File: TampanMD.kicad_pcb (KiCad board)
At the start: 2 copper layers, 50 x 50 mm, 93 parts, among them J1 Conn_01x10, U1 F2800132RHBR, U10 BSC009NE2LS, U11 AMC1301DWVR, U12 TLV62130, U2 UCC27211DRMR, U3 UCC27211DRMR, U4 UCC27211DRMR, U5 BSC009NE2LS, U6 BSC009NE2LS, U7 BSC009NE2LS, U8 BSC009NE2LS, U9 BSC009NE2LS, Y1 X322520MSB4SI

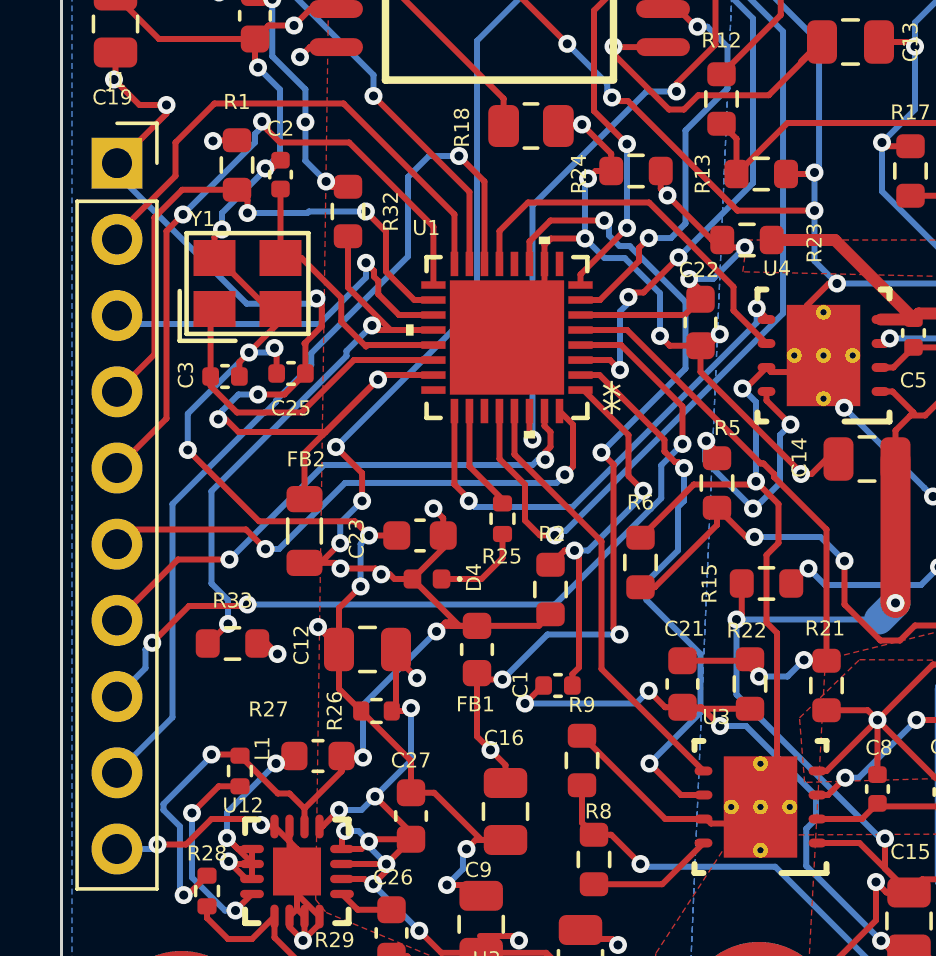
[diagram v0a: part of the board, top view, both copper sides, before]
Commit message: done i guess
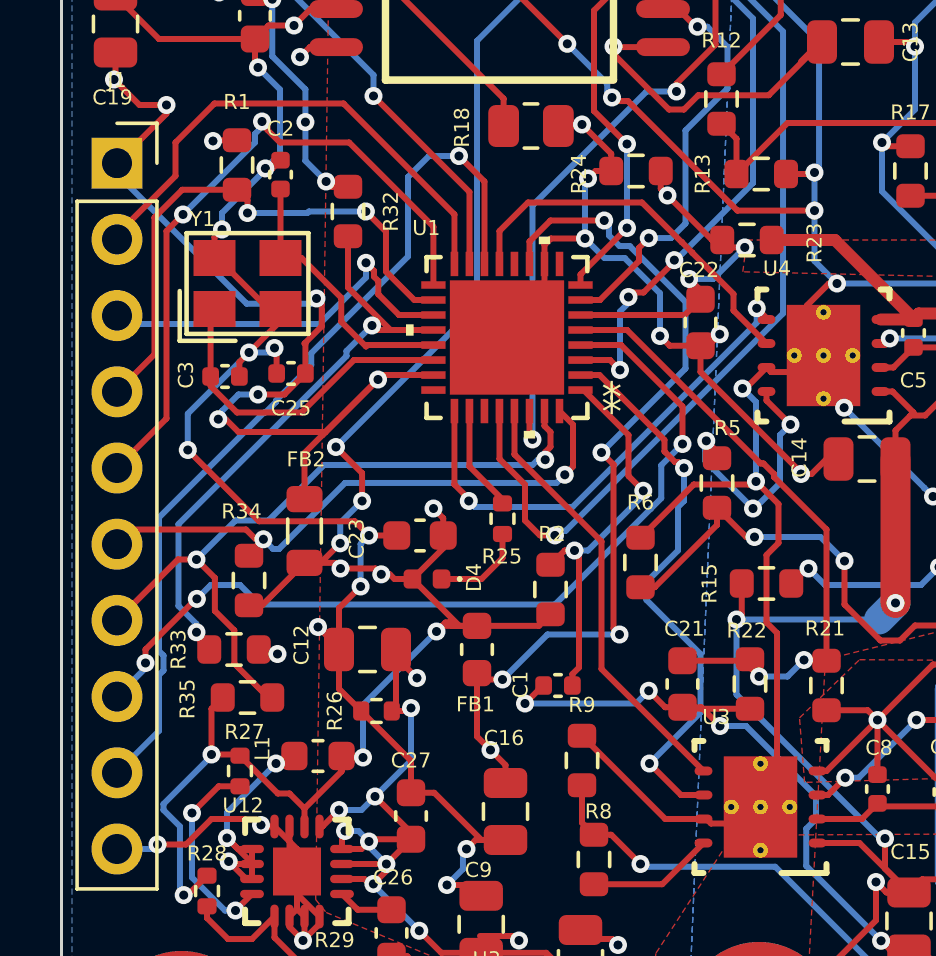
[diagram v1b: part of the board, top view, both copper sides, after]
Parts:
- added R34: 10K, Resistor_SMD:R_0603_1608Metric, F.Cu at (116.9, 79.3)
- added R35: 10K, Resistor_SMD:R_0603_1608Metric, F.Cu at (116.8, 83.2)
- moved R33 0.21 mm to (116.4, 81.7)
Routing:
- net /MCU/I2CB_SCL: track 18.3 -> 24.0 mm
- net 3V3: track 99.1 -> 103.6 mm
- net /MCU/I2CB_SDA: track 18.8 -> 19.6 mm
- net Net-(U1-GPIO32): track 19.5 -> 20.1 mm
- net /MCU/CANA_TX: track 28.8 -> 29.4 mm
